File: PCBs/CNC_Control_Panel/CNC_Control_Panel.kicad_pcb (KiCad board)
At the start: 2 copper layers, 65 x 56 mm, 5 parts, among them P1 Conn_02x20_Odd_Even

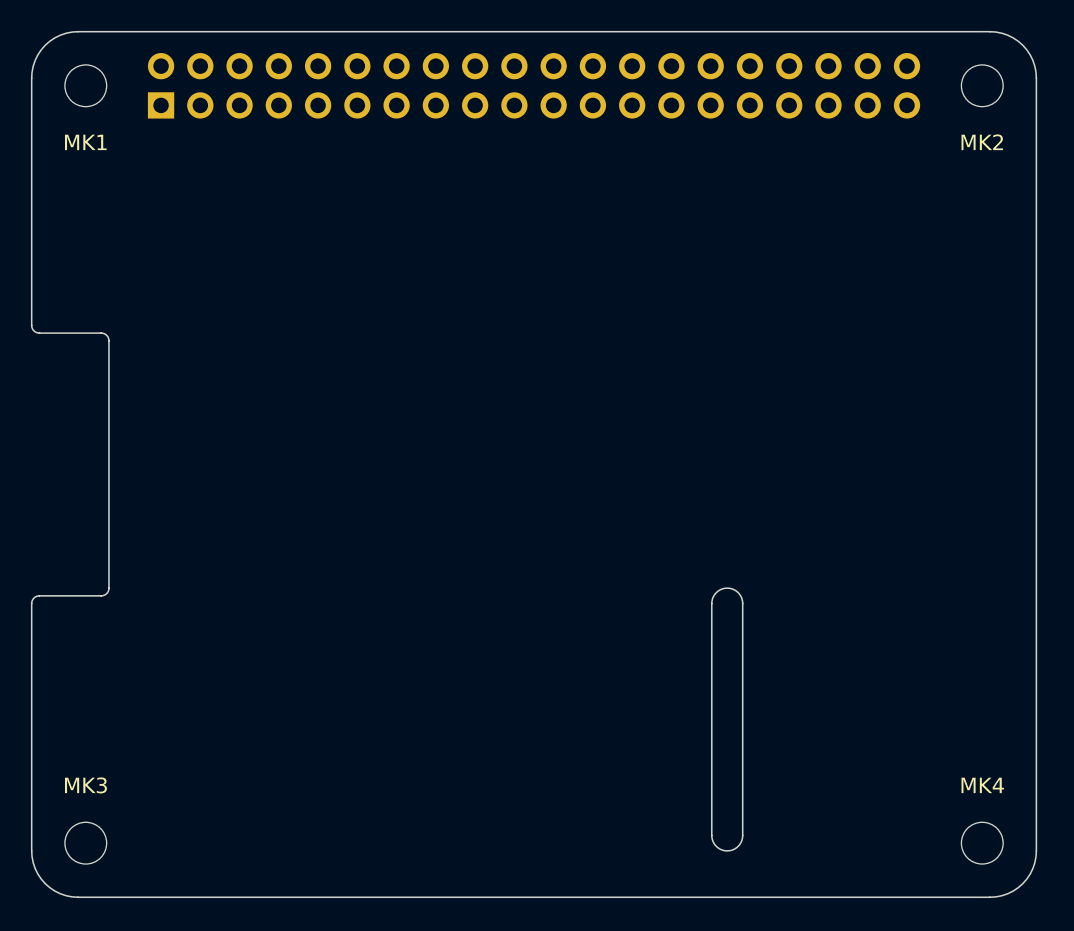
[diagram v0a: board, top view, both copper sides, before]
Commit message: finished schematic and initial layout
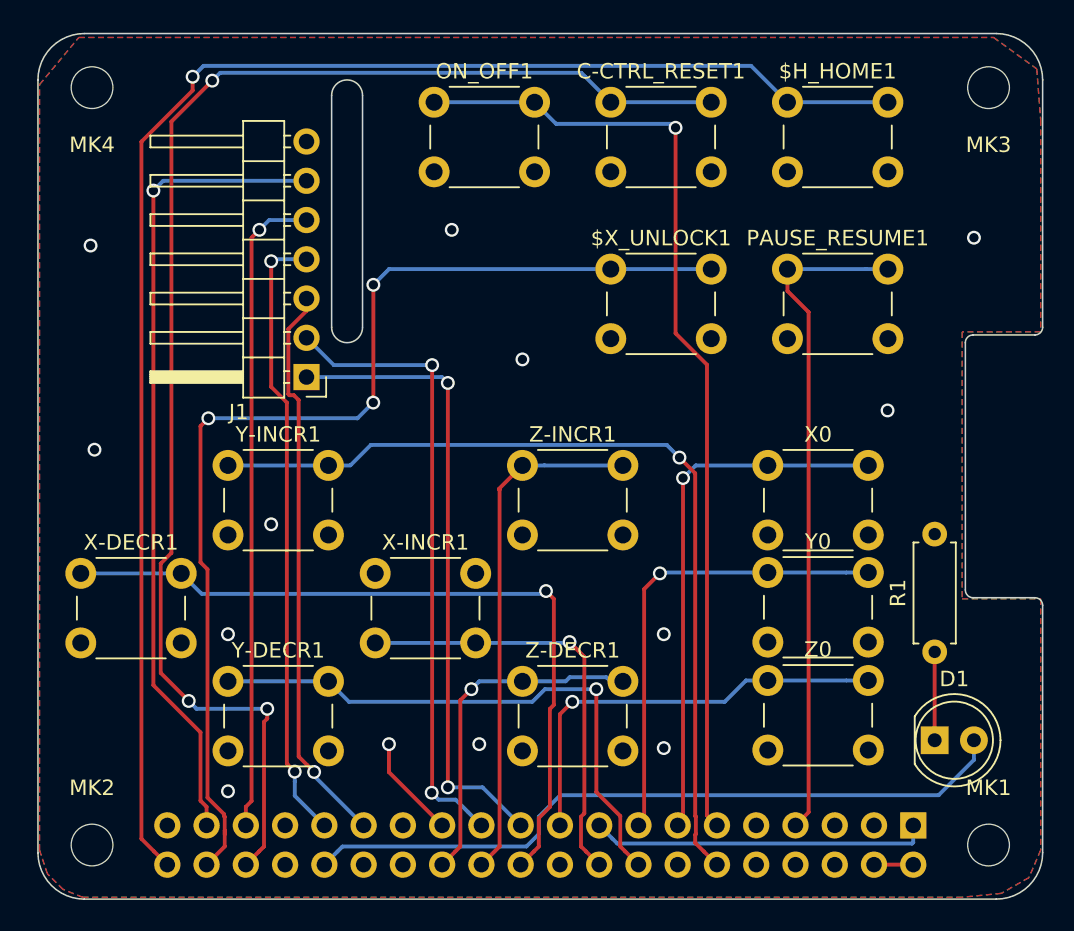
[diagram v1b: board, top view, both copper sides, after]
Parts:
- added $H_HOME1: SW_Push, Button_Switch_THT:SW_PUSH_6mm, F.Cu at (248.9, 98.6)
- added $X_UNLOCK1: SW_Push, Button_Switch_THT:SW_PUSH_6mm, F.Cu at (237.5, 109.4)
- added C-CTRL_RESET1: SW_Push, Button_Switch_THT:SW_PUSH_6mm, F.Cu at (237.5, 98.6)
- added D1: LED, LED_THT:LED_D5.0mm, F.Cu at (258.4, 139.8)
- added J1: Conn_01x07_Male, Connector_PinHeader_2.54mm:PinHeader_1x07_P2.54mm_Horizontal, F.Cu at (217.8, 116.3)
- added ON_OFF1: SW_Push, Button_Switch_THT:SW_PUSH_6mm, F.Cu at (226.0, 98.6)
- added PAUSE_RESUME1: SW_Push, Button_Switch_THT:SW_PUSH_6mm, F.Cu at (248.9, 109.4)
- added R1: R, Resistor_THT:R_Axial_DIN0207_L6.3mm_D2.5mm_P7.62mm_Horizontal, F.Cu at (258.4, 134.1)
- added X-DECR1: SW_Push, Button_Switch_THT:SW_PUSH_6mm, F.Cu at (203.2, 129.0)
- added X-INCR1: SW_Push, Button_Switch_THT:SW_PUSH_6mm, F.Cu at (222.2, 129.0)
- added X0: SW_Push, Button_Switch_THT:SW_PUSH_6mm, F.Cu at (247.6, 122.1)
- added Y-DECR1: SW_Push, Button_Switch_THT:SW_PUSH_6mm, F.Cu at (212.7, 136.0)
- added Y-INCR1: SW_Push, Button_Switch_THT:SW_PUSH_6mm, F.Cu at (212.7, 122.1)
- added Y0: SW_Push, Button_Switch_THT:SW_PUSH_6mm, F.Cu at (247.6, 129.0)
- added Z-DECR1: SW_Push, Button_Switch_THT:SW_PUSH_6mm, F.Cu at (231.8, 136.0)
- added Z-INCR1: SW_Push, Button_Switch_THT:SW_PUSH_6mm, F.Cu at (231.8, 122.1)
- added Z0: SW_Push, Button_Switch_THT:SW_PUSH_6mm, F.Cu at (247.6, 136.0)
- moved MK1 76.3 mm to (261.9, 146.6), turned to 0 degrees
- moved MK3 76.2 mm to (261.9, 97.6), turned to 180 degrees
- moved MK2 75.7 mm to (203.9, 146.6), turned to 0 degrees
- moved MK4 75.5 mm to (203.9, 97.6), turned to 180 degrees
- moved P1 67.4 mm to (257.0, 145.3), turned to 90 degrees
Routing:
- net /GPIO21(SPI1_SCK): track 0.00 -> 99.3 mm, vias 0 -> 1
- net /GPIO16: track 0.00 -> 91.5 mm, vias 0 -> 3
- net /GPIO20(SPI1_MOSI): track 0.00 -> 72.3 mm, vias 0 -> 3
- net /GPIO17(GEN0): track 0.00 -> 62.5 mm, vias 0 -> 1
- net /GPIO18(GEN1)(PWM0): track 0.00 -> 57.5 mm, vias 0 -> 1
- net /GPIO26: track 0.00 -> 52.7 mm, vias 0 -> 1
- net /GPIO25(GEN6): track 0.00 -> 49.5 mm, vias 0 -> 1
- net /GPIO12(PWM0): track 0.00 -> 46.8 mm
- net /GPIO4(GCLK): track 0.00 -> 43.4 mm
- net /GPIO19(SPI1_MISO): track 0.00 -> 42.2 mm, vias 0 -> 1
- net /GPIO9(SPI0_MISO): track 0.00 -> 41.2 mm, vias 0 -> 2
- net /GPIO11(SPI0_SCK): track 0.00 -> 40.6 mm, vias 0 -> 2
- net /GPIO6: track 0.00 -> 40.3 mm, vias 0 -> 2
- net /GPIO23(GEN4): track 0.00 -> 37.2 mm, vias 0 -> 1
- net /GPIO5: track 0.00 -> 36.8 mm, vias 0 -> 1
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- added copper zone on B.Cu, net GND
- added copper zone on F.Cu, net GND
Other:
- outline, holes or cut-outs redrawn
